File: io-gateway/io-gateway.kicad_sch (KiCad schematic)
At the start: 0 parts

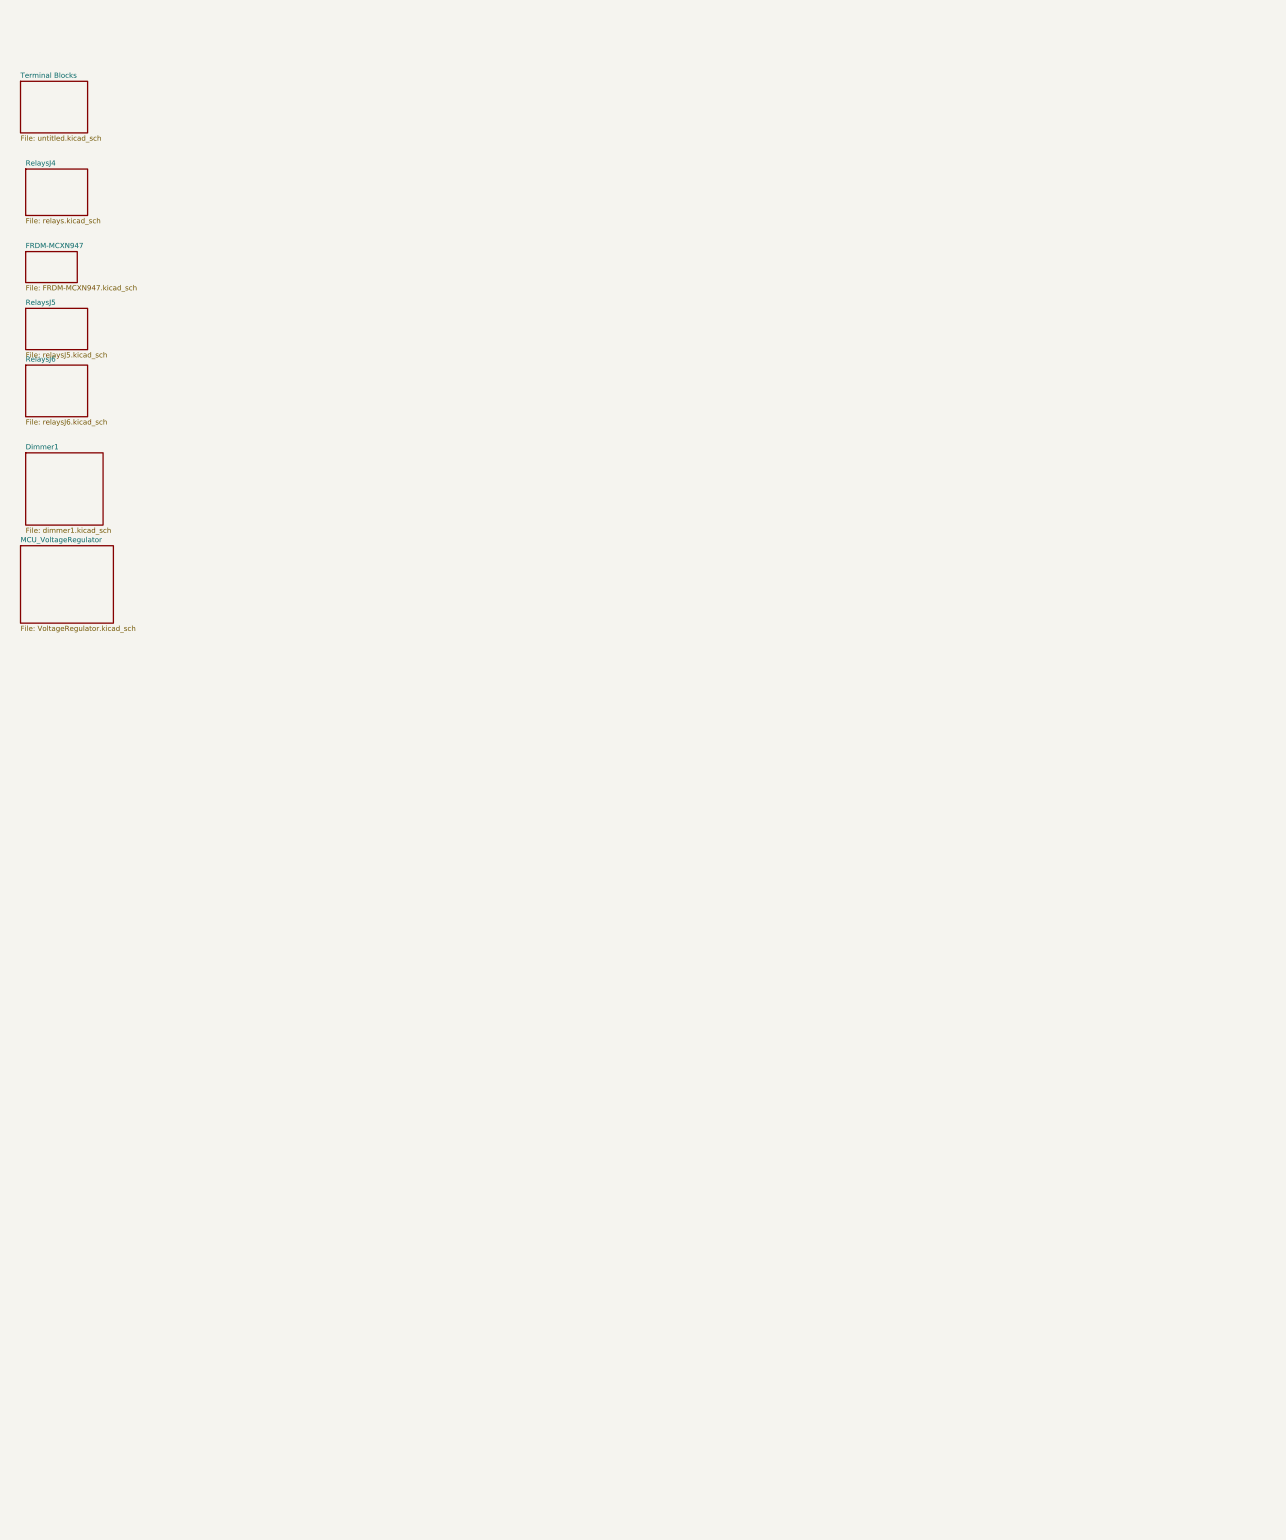
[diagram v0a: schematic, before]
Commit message: temp
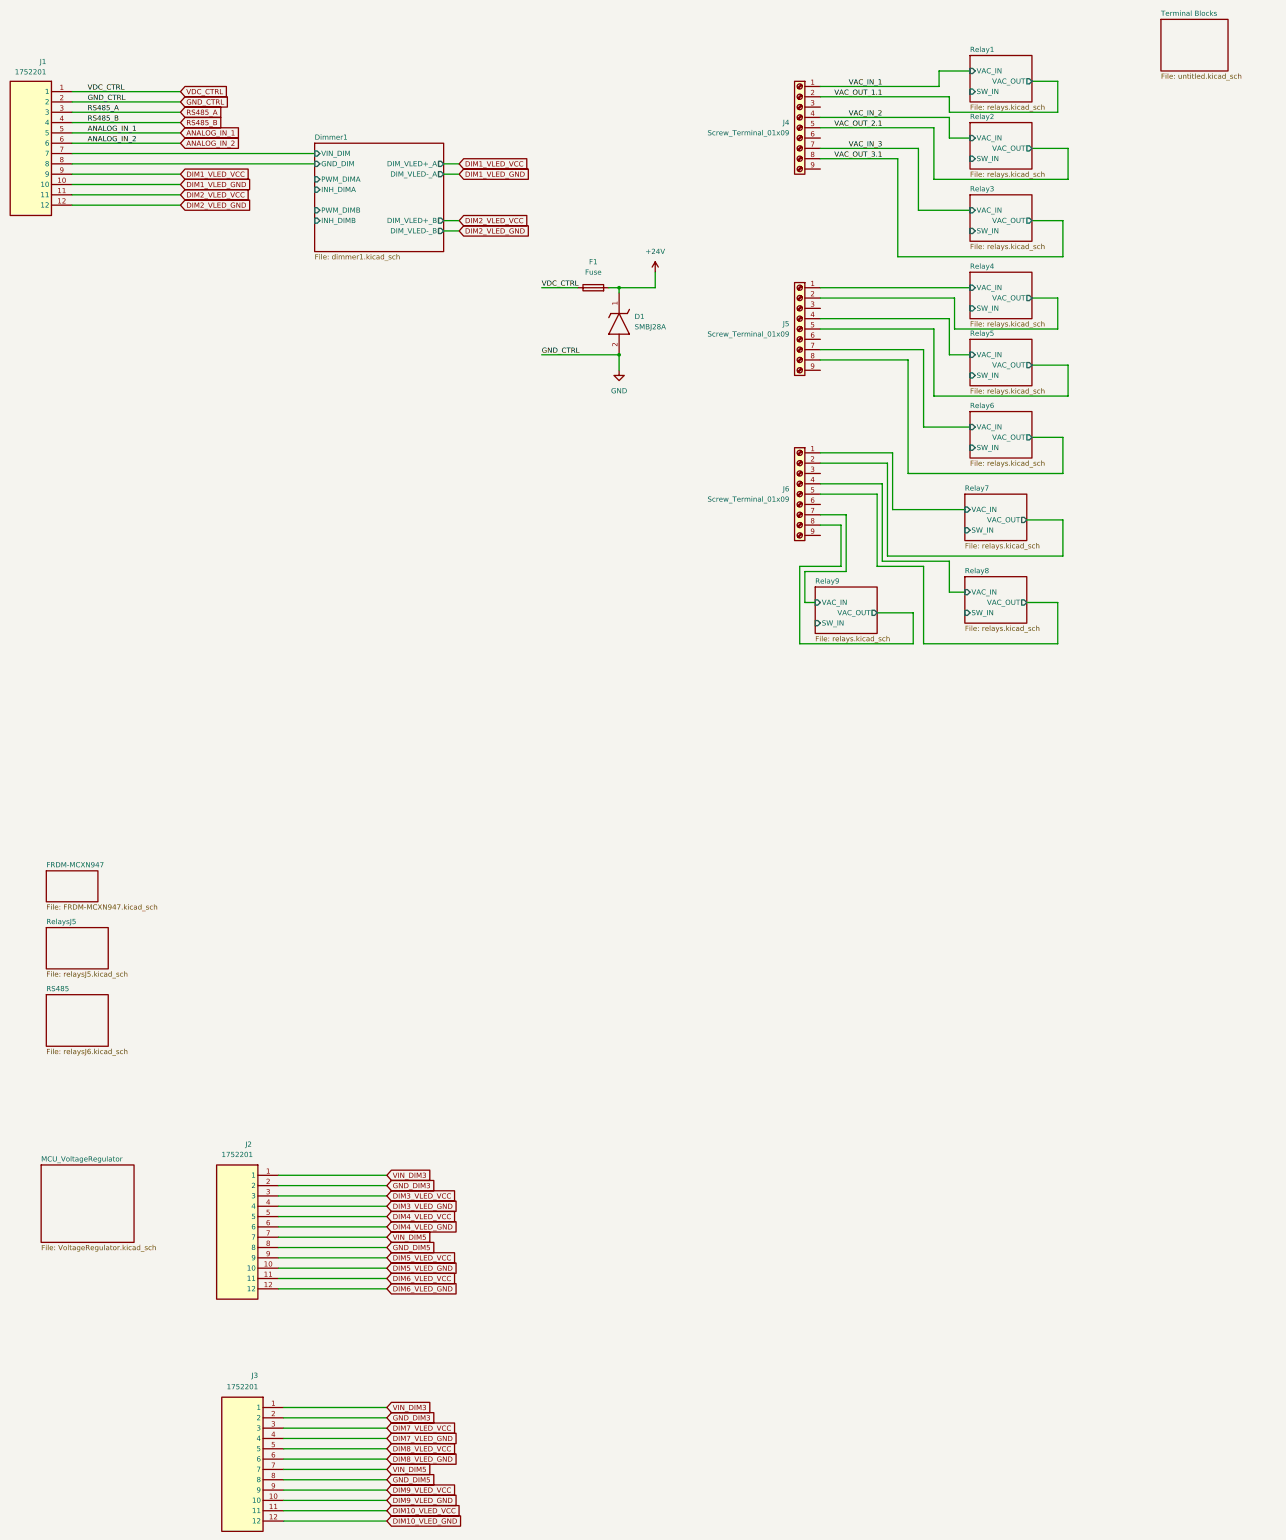
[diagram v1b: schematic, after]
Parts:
- added D1: SMBJ28A, TVS_Diodes:DIOM5436X244N, symbol SMBJ28A:SMBJ28A
- added F1: Fuse, Fuse:Fuseholder_Cylinder-5x20mm_Wuerth_696103101002-SMD_Horizontal_Open, symbol Device:Fuse
- added J1, J2, J3: 1752201, TerminalBlock_Phoenix:1752201, symbol 1752201:1752201
- added J4, J5, J6: Screw_Terminal_01x09, TerminalBlock_TE-Connectivity:TerminalBlock_TE_282836-9_1x09_P5mm_Horizontal, symbol Connector:Screw_Terminal_01x09
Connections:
- new net +24V: D1.1 (K), F1.2
- new net ANALOG_IN_1: J1.5
- new net ANALOG_IN_2: J1.6
- new net DIM10_VLED_GND: J3.12
- new net DIM10_VLED_VCC: J3.11
- new net DIM1_VLED_GND: J1.10
- new net DIM1_VLED_VCC: J1.9
- new net DIM2_VLED_GND: J1.12
- new net DIM2_VLED_VCC: J1.11
- new net DIM3_VLED_GND: J2.4
- new net DIM3_VLED_VCC: J2.3
- new net DIM4_VLED_GND: J2.6
- new net DIM4_VLED_VCC: J2.5
- new net DIM5_VLED_GND: J2.10
- new net DIM5_VLED_VCC: J2.9
- new net DIM6_VLED_GND: J2.12
- new net DIM6_VLED_VCC: J2.11
- new net DIM7_VLED_GND: J3.4
- new net DIM7_VLED_VCC: J3.3
- new net DIM8_VLED_GND: J3.6
- new net DIM8_VLED_VCC: J3.5
- new net DIM9_VLED_GND: J3.10
- new net DIM9_VLED_VCC: J3.9
- new net Dimmer1/GND_DIM: J1.8
- new net Dimmer1/VIN_DIM: J1.7
- new net GND: D1.2 (A), J1.2
- new net GND_DIM3: J2.2, J3.2
- new net GND_DIM5: J2.8, J3.8
- new net RS485_A: J1.3
- new net RS485_B: J1.4
- new net Relay4/VAC_IN: J5.1 (Pin_1)
- new net Relay4/VAC_OUT: J5.2 (Pin_2)
- new net Relay5/VAC_IN: J5.4 (Pin_4)
- new net Relay5/VAC_OUT: J5.5 (Pin_5)
- new net Relay6/VAC_IN: J5.7 (Pin_7)
- new net Relay6/VAC_OUT: J5.8 (Pin_8)
- new net Relay7/VAC_IN: J6.1 (Pin_1)
- new net Relay7/VAC_OUT: J6.2 (Pin_2)
- new net Relay8/VAC_IN: J6.4 (Pin_4)
- new net Relay8/VAC_OUT: J6.5 (Pin_5)
- new net Relay9/VAC_IN: J6.7 (Pin_7)
- new net Relay9/VAC_OUT: J6.8 (Pin_8)
- new net VAC_IN_1: J4.1 (Pin_1)
- new net VAC_IN_2: J4.4 (Pin_4)
- new net VAC_IN_3: J4.7 (Pin_7)
- new net VAC_OUT_1.1: J4.2 (Pin_2)
- new net VAC_OUT_2.1: J4.5 (Pin_5)
- new net VAC_OUT_3.1: J4.8 (Pin_8)
- new net VDC_CTRL: F1.1, J1.1
- new net VIN_DIM3: J2.1, J3.1
- new net VIN_DIM5: J2.7, J3.7
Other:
- sheet RelaysJ4 renamed Relay1
- sheet RelaysJ6 renamed RS485
- added sheet Relay2 (relays.kicad_sch)
- added sheet Relay3 (relays.kicad_sch)
- added sheet Relay4 (relays.kicad_sch)
- added sheet Relay5 (relays.kicad_sch)
- added sheet Relay6 (relays.kicad_sch)
- added sheet Relay7 (relays.kicad_sch)
- added sheet Relay8 (relays.kicad_sch)
- added sheet Relay9 (relays.kicad_sch)
- sheet Dimmer1 ports: added DIM_VLED+_A, DIM_VLED+_B, DIM_VLED-_A, DIM_VLED-_B, GND_DIM, INH_DIMA, INH_DIMB, PWM_DIMA, PWM_DIMB, VIN_DIM; removed none
- sheet Relay1 ports: added SW_IN, VAC_IN, VAC_OUT; removed none
